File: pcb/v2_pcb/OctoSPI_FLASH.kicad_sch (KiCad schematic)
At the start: 5 parts, among them U5 MX25U51279GXDR00

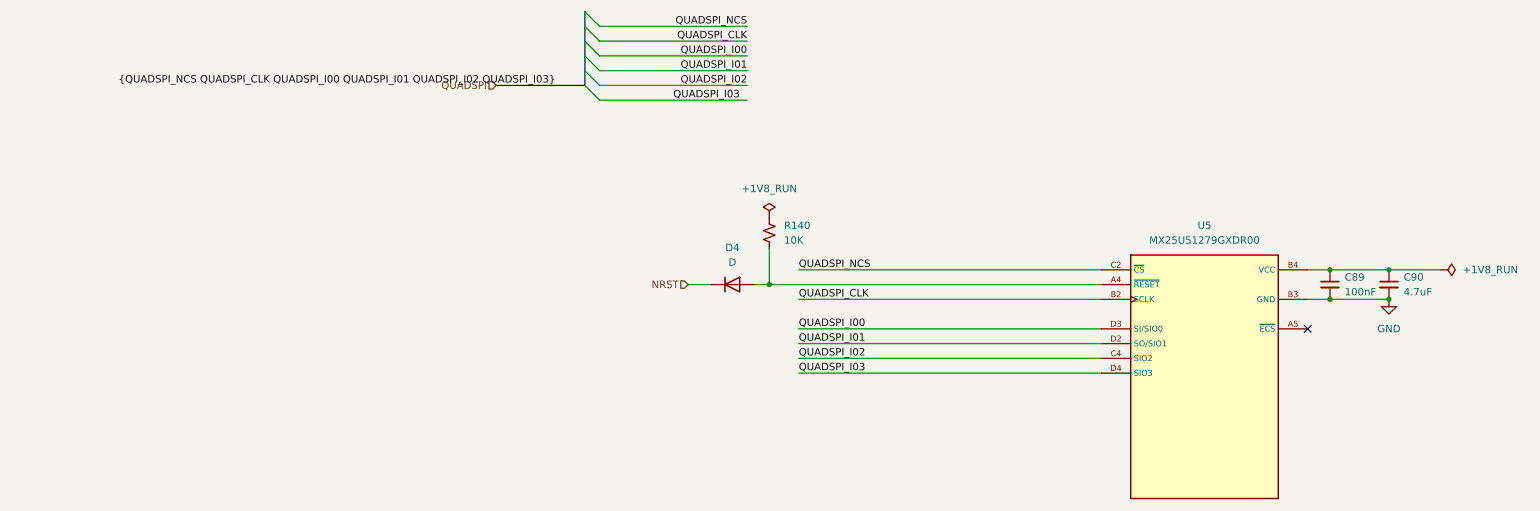
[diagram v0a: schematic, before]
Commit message: pcb done
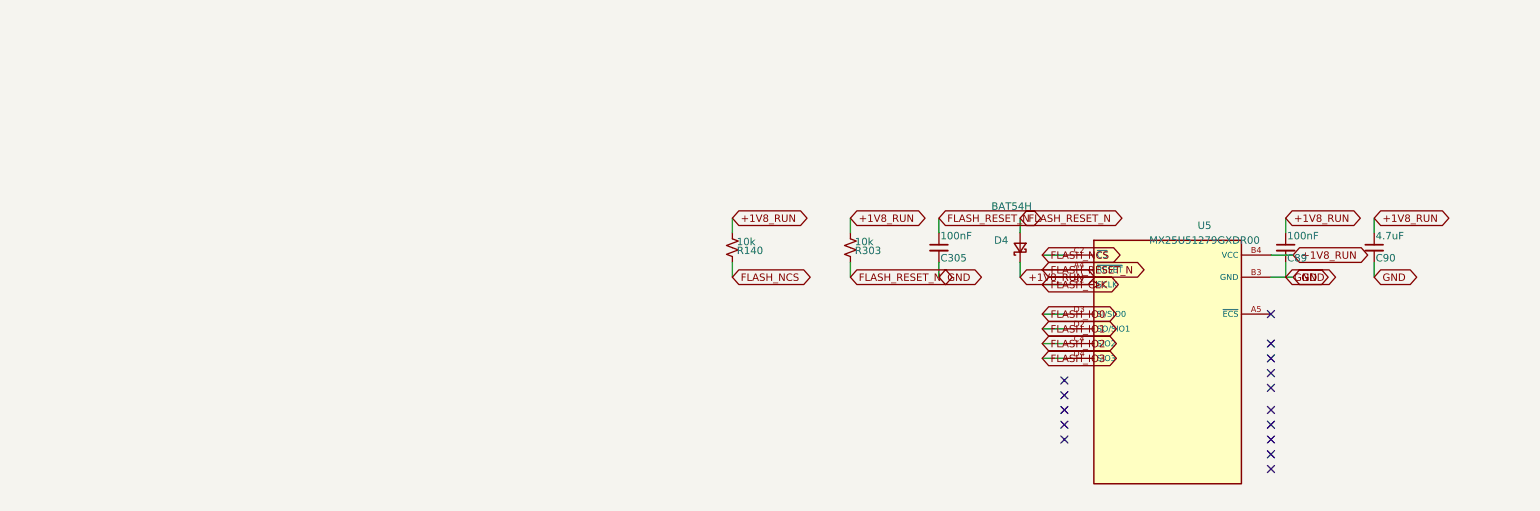
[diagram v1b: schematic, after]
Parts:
- removed D4: D, symbol Device:D
- added C305: 100nF, Capacitor_SMD:C_0402_1005Metric, symbol Device:C_Small
- added D4: BAT54H, Diode_SMD:D_SOD-323, symbol Device:D_Schottky_Small
- added R303: 10k, Resistor_SMD:R_0402_1005Metric, symbol Device:R_Small_US
- C89: footprint (none) -> Capacitor_SMD:C_0402_1005Metric
- C90: footprint (none) -> Capacitor_SMD:C_0603_1608Metric
- R140: value 10K -> 10k; footprint (none) -> Resistor_SMD:R_0402_1005Metric
- U5: footprint MX66UW1G45GXDI00:BGA24C100P5X5_800X600X120 -> noob:BGA24C100P5X5_800X600X120; MPN (none) -> MX25U51279GXDR00; Manufacturer (none) -> Macronix
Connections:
- net QUADSPI_NCS is gone; now on net FLASH_NCS: U5.C2 (~{CS})
- net GND: now also C305.2
- net FLASH_NCS: now reaches R140.2
- net FLASH_NCS: no longer U5.A4 (~{RESET})
- net +1V8_RUN: now reaches C89.1, C90.1, U5.B4 (VCC)
- net +1V8_RUN: now also R140.1, D4.1 (K), R303.1
- net QUADSPI_CLK renamed FLASH_CLK
- net QUADSPI_I00 renamed FLASH_IO0
- net QUADSPI_I01 renamed FLASH_IO1
- net QUADSPI_I02 renamed FLASH_IO2
- net QUADSPI_I03 renamed FLASH_IO3
- new net FLASH_RESET_N: C305.1, D4.2 (A), R303.2, U5.A4 (~{RESET})
- no-connect marks 1 -> 15
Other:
- moved on the sheet: U5
